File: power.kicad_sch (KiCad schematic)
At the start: 8 parts, among them U1 NCP1117-3.3_SOT223

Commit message: Initial commit
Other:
- title: FRANK -> MiniFRANK
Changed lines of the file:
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@@
 	(paper "A4")
 	(title_block
-		(title "FRANK")
-		(date "2024-12-15")
+		(title "MiniFRANK")
+		(date "2025-01-12")
 		(rev "2.0")
 		(company "Mikhail Matveev")
-		(comment 1 "https://github.com/xtremespb/frank2")
+		(comment 1 "https://github.com/xtremespb/frank")
 	)
 	(junction

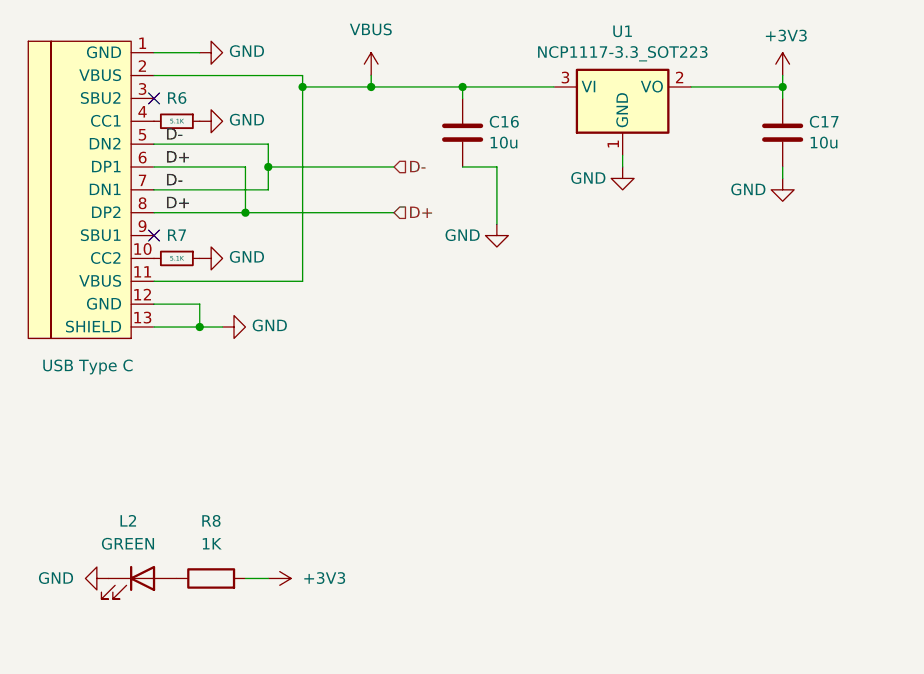
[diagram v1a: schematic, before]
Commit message: Minor updates
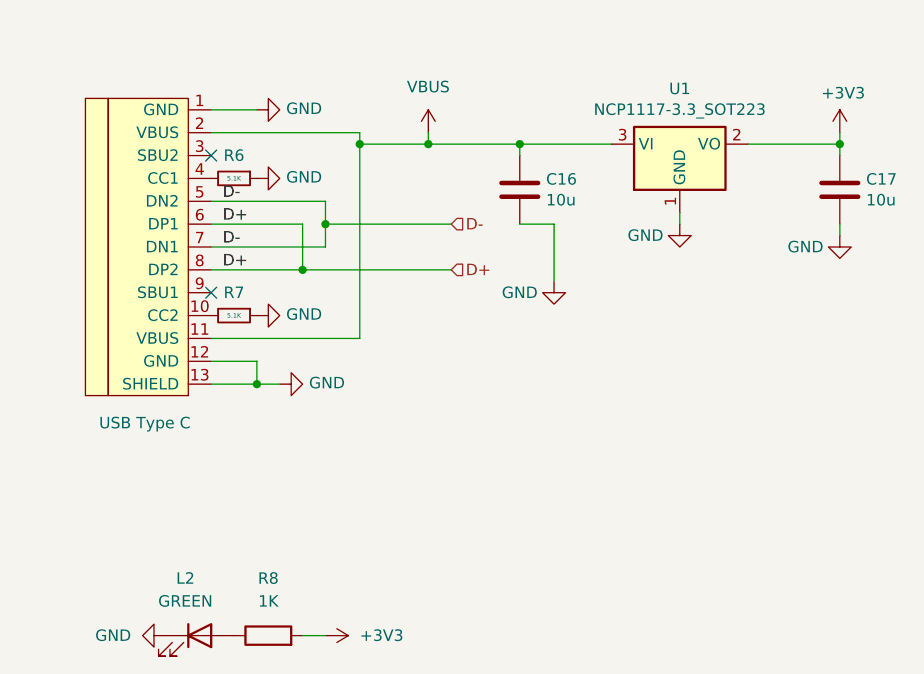
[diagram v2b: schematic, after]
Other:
- moved on the sheet: C16, C17, L2, R6, R7, R8, U1
